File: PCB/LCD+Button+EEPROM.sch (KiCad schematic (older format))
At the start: 17 parts, among them J2 Conn_01x03, J3 Conn_01x04, J4 Conn_01x03, J5 Conn_01x04, J6 Conn_01x04, SW1 B1, SW2 B2, SW3 B3, SW4 B4, SW5 B5, SW6 B6, U4 24LC256

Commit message: Footprint Assigned
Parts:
- C18: footprint (none) -> Capacitor_SMD:C_0805_2012Metric
- J2, J4: footprint (none) -> Connector_PinHeader_2.54mm:PinHeader_1x03_P2.54mm_Vertical
- J3, J5, J6: footprint (none) -> Connector_PinHeader_2.54mm:PinHeader_1x04_P2.54mm_Vertical
- LCD1: footprint (none) -> Kicad Library:OLED_I2C_128x64
- R10, R11: footprint (none) -> Resistor_SMD:R_0805_2012Metric
- RESET1, SW1, SW2, SW3, SW4, SW5, SW6: footprint (none) -> Kicad Library:Push_button_silicon_mute
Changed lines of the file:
@@
 F 0 "RESET1" H 5650 4000 50  0000 R CNN
 F 1 "RESET" H 5875 3950 50  0001 R CNN
-F 2 "" H 5525 4050 50  0001 C CNN
+F 2 "Kicad Library:Push_button_silicon_mute" H 5525 4050 50  0001 C CNN
 F 3 "~" H 5525 4050 50  0001 C CNN
 	1    5525 3850
@@
 F 0 "SW1" H 5600 4250 50  0000 R CNN
 F 1 "B1" H 5725 4200 50  0001 R CNN
-F 2 "" H 5525 4300 50  0001 C CNN
+F 2 "Kicad Library:Push_button_silicon_mute" H 5525 4300 50  0001 C CNN
 F 3 "~" H 5525 4300 50  0001 C CNN
 	1    5525 4100
@@
 F 0 "SW2" H 5600 4500 50  0000 R CNN
 F 1 "B2" H 5725 4450 50  0001 R CNN
-F 2 "" H 5525 4550 50  0001 C CNN
+F 2 "Kicad Library:Push_button_silicon_mute" H 5525 4550 50  0001 C CNN
 F 3 "~" H 5525 4550 50  0001 C CNN
 	1    5525 4350
@@
 F 0 "SW3" H 5600 4750 50  0000 R CNN
 F 1 "B3" H 5725 4700 50  0001 R CNN
-F 2 "" H 5525 4800 50  0001 C CNN
+F 2 "Kicad Library:Push_button_silicon_mute" H 5525 4800 50  0001 C CNN
 F 3 "~" H 5525 4800 50  0001 C CNN
 	1    5525 4600
@@
 F 0 "SW4" H 4625 4175 50  0000 R CNN
 F 1 "B4" H 4725 4125 50  0001 R CNN
-F 2 "" H 4525 4225 50  0001 C CNN
+F 2 "Kicad Library:Push_button_silicon_mute" H 4525 4225 50  0001 C CNN
 F 3 "~" H 4525 4225 50  0001 C CNN
 	1    4525 4025
@@
 F 0 "SW5" H 4625 4425 50  0000 R CNN
 F 1 "B5" H 4725 4375 50  0001 R CNN
-F 2 "" H 4525 4475 50  0001 C CNN
+F 2 "Kicad Library:Push_button_silicon_mute" H 4525 4475 50  0001 C CNN
 F 3 "~" H 4525 4475 50  0001 C CNN
 	1    4525 4275
@@
 F 0 "SW6" H 4625 4675 50  0000 R CNN
 F 1 "B6" H 4725 4625 50  0001 R CNN
-F 2 "" H 4525 4725 50  0001 C CNN
+F 2 "Kicad Library:Push_button_silicon_mute" H 4525 4725 50  0001 C CNN
 F 3 "~" H 4525 4725 50  0001 C CNN
 	1    4525 4525
@@
 F 0 "J3" H 6605 3896 50  0000 L CNN
 F 1 "Conn_01x04" H 6605 3851 50  0001 L CNN
-F 2 "" H 6525 3950 50  0001 C CNN
+F 2 "Connector_PinHeader_2.54mm:PinHeader_1x04_P2.54mm_Vertical" H 6525 3950 50  0001 C CNN
 F 3 "~" H 6525 3950 50  0001 C CNN
 	1    6525 3950
@@
 F 0 "J2" H 3750 4125 50  0000 C CNN
 F 1 "Conn_01x03" H 3518 3891 50  0001 C CNN
-F 2 "" H 3600 4125 50  0001 C CNN
+F 2 "Connector_PinHeader_2.54mm:PinHeader_1x03_P2.54mm_Vertical" H 3600 4125 50  0001 C CNN
 F 3 "~" H 3600 4125 50  0001 C CNN
 	1    3600 4125
@@
 AR Path="/5F734488" Ref="#PWR?"  Part="1"
 AR Path="/5F584CC7/5F734488" Ref="#PWR?"  Part="1"
-AR Path="/5F7200D9/5F734488" Ref="#PWR03"  Part="1"
-F 0 "#PWR03" H 5025 4350 50  0001 C CNN
+AR Path="/5F7200D9/5F734488" Ref="#PWR0101"  Part="1"
+F 0 "#PWR0101" H 5025 4350 50  0001 C CNN
 F 1 "GND" H 5030 4427 50  0000 C CNN
 F 2 "" H 5025 4600 50  0001 C CNN
@@
 F 0 "J5" V 5100 5175 50  0000 C CNN
 F 1 "Conn_01x04" V 5100 5175 50  0001 C CNN
-F 2 "" H 5000 5200 50  0001 C CNN
+F 2 "Connector_PinHeader_2.54mm:PinHeader_1x04_P2.54mm_Vertical" H 5000 5200 50  0001 C CNN
 F 3 "~" H 5000 5200 50  0001 C CNN
 	1    5000 5200
@@
 AR Path="/5F647117" Ref="#PWR?"  Part="1"
 AR Path="/5F584CC7/5F647117" Ref="#PWR?"  Part="1"
-AR Path="/5F7200D9/5F647117" Ref="#PWR02"  Part="1"
-F 0 "#PWR02" H 4900 5425 50  0001 C CNN
+AR Path="/5F7200D9/5F647117" Ref="#PWR0102"  Part="1"
+F 0 "#PWR0102" H 4900 5425 50  0001 C CNN
 F 1 "GND" H 4905 5502 50  0000 C CNN
 F 2 "" H 4900 5675 50  0001 C CNN
@@
 F 0 "J4" V 4650 5200 50  0000 C CNN
 F 1 "Conn_01x03" H 4468 4966 50  0001 C CNN
-F 2 "" H 4550 5200 50  0001 C CNN
+F 2 "Connector_PinHeader_2.54mm:PinHeader_1x03_P2.54mm_Vertical" H 4550 5200 50  0001 C CNN
 F 3 "~" H 4550 5200 50  0001 C CNN
 	1    4550 5200
@@
 F 0 "J6" V 5650 5125 50  0000 L CNN
 F 1 "Conn_01x04" H 5630 5101 50  0001 L CNN
-F 2 "" H 5550 5200 50  0001 C CNN
+F 2 "Connector_PinHeader_2.54mm:PinHeader_1x04_P2.54mm_Vertical" H 5550 5200 50  0001 C CNN
 F 3 "~" H 5550 5200 50  0001 C CNN
 	1    5550 5200
@@
 F 0 "R10" H 5575 2650 50  0000 L CNN
 F 1 "2K2" V 5525 2550 50  0000 L CNN
-F 2 "" V 5455 2625 50  0001 C CNN
+F 2 "Resistor_SMD:R_0805_2012Metric" V 5455 2625 50  0001 C CNN
 F 3 "~" H 5525 2625 50  0001 C CNN
 	1    5525 2625
@@
 F 0 "R11" H 5850 2650 50  0000 L CNN
 F 1 "2K2" V 5800 2550 50  0000 L CNN
-F 2 "" V 5730 2625 50  0001 C CNN
+F 2 "Resistor_SMD:R_0805_2012Metric" V 5730 2625 50  0001 C CNN
 F 3 "~" H 5800 2625 50  0001 C CNN
 	1    5800 2625
@@
 F 0 "C18" H 4315 2971 50  0000 L CNN
 F 1 "100nF" H 4315 2880 50  0000 L CNN
-F 2 "" H 4238 2775 50  0001 C CNN
+F 2 "Capacitor_SMD:C_0805_2012Metric" H 4238 2775 50  0001 C CNN
 F 3 "~" H 4200 2925 50  0001 C CNN
 	1    4200 2925
@@
 F 0 "LCD1" V 3650 2775 50  0000 C CNN
 F 1 "LCD" V 3650 2775 50  0001 C CNN
-F 2 "" H 3550 2800 50  0001 C CNN
+F 2 "Kicad Library:OLED_I2C_128x64" H 3550 2800 50  0001 C CNN
 F 3 "~" H 3550 2800 50  0001 C CNN
 	1    3550 2800

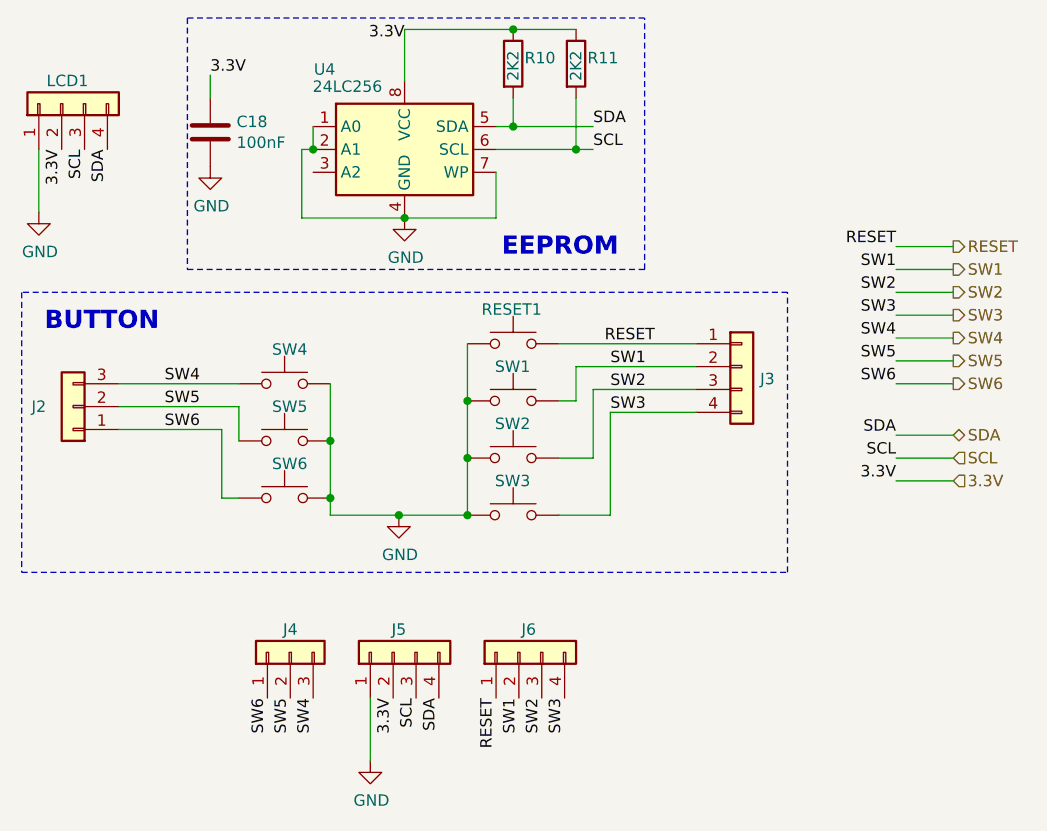
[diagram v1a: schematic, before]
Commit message: Circuit fix (Kicad)
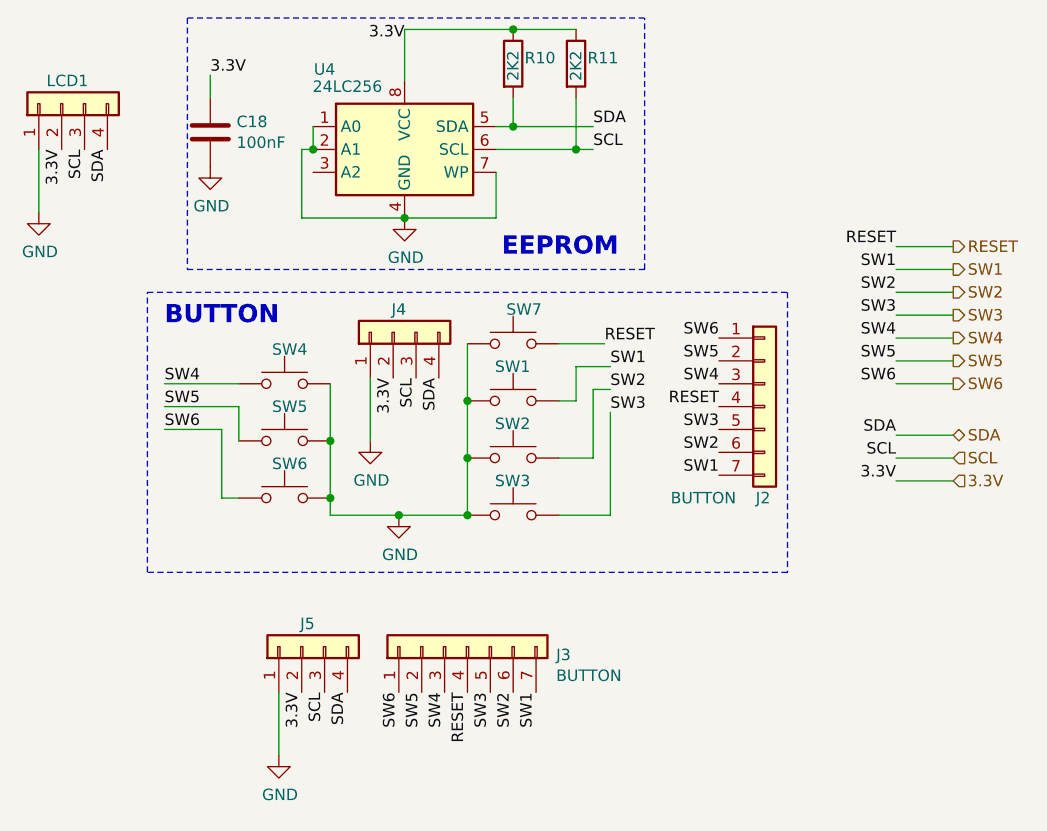
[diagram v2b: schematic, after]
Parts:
- removed J2, J4: Conn_01x03, Connector_PinHeader_2.54mm:PinHeader_1x03_P2.54mm_Vertical, symbol Connector_Generic:Conn_01x03
- removed J3, J6: Conn_01x04, Connector_PinHeader_2.54mm:PinHeader_1x04_P2.54mm_Vertical, symbol Connector_Generic:Conn_01x04
- added J2: BUTTON, Connector_PinSocket_2.54mm:PinSocket_1x07_P2.54mm_Vertical, symbol Connector_Generic:Conn_01x07
- added J3: BUTTON, Connector_PinHeader_2.54mm:PinHeader_1x07_P2.54mm_Vertical, symbol Connector_Generic:Conn_01x07
- added J4: Conn_01x04, Connector_PinHeader_2.54mm:PinHeader_1x04_P2.54mm_Vertical, symbol Connector_Generic:Conn_01x04
- J5: footprint Connector_PinHeader_2.54mm:PinHeader_1x04_P2.54mm_Vertical -> Connector_PinSocket_2.54mm:PinSocket_1x04_P2.54mm_Vertical
- renumbered RESET1 to SW7
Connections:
- net 3.3V: now also J4.2 (Pin_2)
- net GND: now also J4.1 (Pin_1)
- net RESET: now also J2.4 (Pin_4), J3.4 (Pin_4)
- net SCL: now also J4.3 (Pin_3)
- net SDA: now also J4.4 (Pin_4)
- net SW1: now also J2.7 (Pin_7), J3.7 (Pin_7)
- net SW2: now also J2.6 (Pin_6), J3.6 (Pin_6)
- net SW3: now also J2.5 (Pin_5), J3.5 (Pin_5)
- net SW4: now also J2.3 (Pin_3), J3.3 (Pin_3)
- net SW5: now also J2.2 (Pin_2), J3.2 (Pin_2)
- net SW6: now also J2.1 (Pin_1), J3.1 (Pin_1)
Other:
- moved on the sheet: J5
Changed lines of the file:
@@
 P 5525 3850
 AR Path="/5F727D85" Ref="SW?"  Part="1"
-AR Path="/5F7200D9/5F727D85" Ref="RESET1"  Part="1"
-F 0 "RESET1" H 5650 4000 50  0000 R CNN
+AR Path="/5F7200D9/5F727D85" Ref="SW7"  Part="1"
+F 0 "SW7" H 5650 4000 50  0000 R CNN
 F 1 "RESET" H 5875 3950 50  0001 R CNN
 F 2 "Kicad Library:Push_button_silicon_mute" H 5525 4050 50  0001 C CNN
@@
 	1    0    0    -1
 $EndComp
-$Comp
-L Connector_Generic:Conn_01x04 J?
-U 1 1 5F727DAF
-P 6525 3950
-AR Path="/5F727DAF" Ref="J?"  Part="1"
-AR Path="/5F7200D9/5F727DAF" Ref="J3"  Part="1"
-F 0 "J3" H 6605 3896 50  0000 L CNN
-F 1 "Conn_01x04" H 6605 3851 50  0001 L CNN
-F 2 "Connector_PinHeader_2.54mm:PinHeader_1x04_P2.54mm_Vertical" H 6525 3950 50  0001 C CNN
-F 3 "~" H 6525 3950 50  0001 C CNN
-	1    6525 3950
-	1    0    0    -1
-$EndComp
-Wire Wire Line
-	5725 3850 6325 3850
 Wire Wire Line
 	5725 4100 5800 4100
@@
 	5800 4100 5800 3950
 Wire Wire Line
-	5800 3950 6325 3950
-Wire Wire Line
 	5725 4350 5875 4350
 Wire Wire Line
 	5875 4350 5875 4050
 Wire Wire Line
-	5875 4050 6325 4050
-Wire Wire Line
 	5725 4600 5950 4600
 Wire Wire Line
 	5950 4600 5950 4150
 Wire Wire Line
-	5950 4150 6325 4150
-$Comp
-L Connector_Generic:Conn_01x03 J2
-U 1 1 5F72E5D5
-P 3600 4125
-F 0 "J2" H 3750 4125 50  0000 C CNN
-F 1 "Conn_01x03" H 3518 3891 50  0001 C CNN
-F 2 "Connector_PinHeader_2.54mm:PinHeader_1x03_P2.54mm_Vertical" H 3600 4125 50  0001 C CNN
-F 3 "~" H 3600 4125 50  0001 C CNN
-	1    3600 4125
-	-1   0    0    1
-$EndComp
-Wire Wire Line
-	4325 4025 3800 4025
-Wire Wire Line
-	3800 4125 4325 4125
-Wire Wire Line
 	4325 4125 4325 4275
-Wire Wire Line
-	3800 4225 4250 4225
 Wire Wire Line
 	4250 4225 4250 4525
@@
 L Connector_Generic:Conn_01x04 J?
 U 1 1 5F647111
-P 5000 5200
+P 4600 5175
 AR Path="/5F647111" Ref="J?"  Part="1"
 AR Path="/5F7200D9/5F647111" Ref="J5"  Part="1"
-F 0 "J5" V 5100 5175 50  0000 C CNN
-F 1 "Conn_01x04" V 5100 5175 50  0001 C CNN
-F 2 "Connector_PinHeader_2.54mm:PinHeader_1x04_P2.54mm_Vertical" H 5000 5200 50  0001 C CNN
-F 3 "~" H 5000 5200 50  0001 C CNN
-	1    5000 5200
+F 0 "J5" V 4700 5150 50  0000 C CNN
+F 1 "Conn_01x04" V 4700 5150 50  0001 C CNN
+F 2 "Connector_PinSocket_2.54mm:PinSocket_1x04_P2.54mm_Vertical" H 4600 5175 50  0001 C CNN
+F 3 "~" H 4600 5175 50  0001 C CNN
+	1    4600 5175
 	0    -1   -1   0
 $EndComp
@@
 L power:GND #PWR?
 U 1 1 5F647117
-P 4900 5675
+P 4500 5650
 AR Path="/5F647117" Ref="#PWR?"  Part="1"
 AR Path="/5F584CC7/5F647117" Ref="#PWR?"  Part="1"
 AR Path="/5F7200D9/5F647117" Ref="#PWR0102"  Part="1"
-F 0 "#PWR0102" H 4900 5425 50  0001 C CNN
-F 1 "GND" H 4905 5502 50  0000 C CNN
-F 2 "" H 4900 5675 50  0001 C CNN
-F 3 "" H 4900 5675 50  0001 C CNN
-	1    4900 5675
-	1    0    0    -1
-$EndComp
-Wire Wire Line
-	4900 5400 4900 5675
+F 0 "#PWR0102" H 4500 5400 50  0001 C CNN
+F 1 "GND" H 4505 5477 50  0000 C CNN
+F 2 "" H 4500 5650 50  0001 C CNN
+F 3 "" H 4500 5650 50  0001 C CNN
+	1    4500 5650
+	1    0    0    -1
+$EndComp
+Wire Wire Line
+	4500 5375 4500 5650
 Text HLabel 7450 4450 2    50   Input ~ 0
 3.3V
@@
 Text HLabel 7450 4250 2    50   BiDi ~ 0
 SDA
-$Comp
-L Connector_Generic:Conn_01x03 J4
-U 1 1 5F64A1B9
-P 4550 5200
-F 0 "J4" V 4650 5200 50  0000 C CNN
-F 1 "Conn_01x03" H 4468 4966 50  0001 C CNN
-F 2 "Connector_PinHeader_2.54mm:PinHeader_1x03_P2.54mm_Vertical" H 4550 5200 50  0001 C CNN
-F 3 "~" H 4550 5200 50  0001 C CNN
-	1    4550 5200
-	0    -1   -1   0
-$EndComp
-Text Label 4650 5400 3    50   ~ 0
+Text Label 5225 5375 3    50   ~ 0
 SW4
-Text Label 4550 5400 3    50   ~ 0
+Text Label 5125 5375 3    50   ~ 0
 SW5
-Text Label 4450 5400 3    50   ~ 0
+Text Label 5025 5375 3    50   ~ 0
 SW6
-$Comp
-L Connector_Generic:Conn_01x04 J?
-U 1 1 5F64BF4F
-P 5550 5200
-AR Path="/5F64BF4F" Ref="J?"  Part="1"
-AR Path="/5F7200D9/5F64BF4F" Ref="J6"  Part="1"
-F 0 "J6" V 5650 5125 50  0000 L CNN
-F 1 "Conn_01x04" H 5630 5101 50  0001 L CNN
-F 2 "Connector_PinHeader_2.54mm:PinHeader_1x04_P2.54mm_Vertical" H 5550 5200 50  0001 C CNN
-F 3 "~" H 5550 5200 50  0001 C CNN
-	1    5550 5200
-	0    -1   -1   0
-$EndComp
-Text Label 5450 5400 3    50   ~ 0
+Text Label 5325 5375 3    50   ~ 0
 RESET
-Text Label 5550 5400 3    50   ~ 0
+Text Label 5625 5375 3    50   ~ 0
 SW1
-Text Label 5650 5400 3    50   ~ 0
+Text Label 5525 5375 3    50   ~ 0
 SW2
-Text Label 5750 5400 3    50   ~ 0
+Text Label 5425 5375 3    50   ~ 0
 SW3
 $Comp
@@
 Text Label 5875 3000 0    50   ~ 0
 SCL
-Text Label 5000 5400 3    50   ~ 0
-3.3V
-Text Label 5100 5400 3    50   ~ 0
+Text Label 4600 5375 3    50   ~ 0
+3.3V
+Text Label 4700 5375 3    50   ~ 0
 SCL
-Text Label 5200 5400 3    50   ~ 0
+Text Label 4800 5375 3    50   ~ 0
 SDA
 $Comp
@@
 Text Label 3750 3000 3    50   ~ 0
 SDA
-Wire Notes Line
-	6725 3625 3375 3625
-Wire Notes Line
-	3375 3625 3375 4850
-Wire Notes Line
-	3375 4850 6725 4850
-Wire Notes Line
-	6725 4850 6725 3625
-Text Notes 3475 3800 0    79   ~ 16
+Text Notes 4000 3775 0    79   ~ 16
 BUTTON
+$Comp
+L Connector_Generic:Conn_01x07 J3
+U 1 1 5F6D5D8E
+P 5325 5175
+F 0 "J3" V 5289 4787 50  0000 R CNN
+F 1 "BUTTON" V 5198 4787 50  0000 R CNN
+F 2 "Connector_PinHeader_2.54mm:PinHeader_1x07_P2.54mm_Vertical" H 5325 5175 50  0001 C CNN
+F 3 "~" H 5325 5175 50  0001 C CNN
+	1    5325 5175
+	0    -1   -1   0
+$EndComp
+Text Label 6425 4025 2    50   ~ 0
+SW4
+Text Label 6425 3925 2    50   ~ 0
+SW5
+Text Label 6425 3825 2    50   ~ 0
+SW6
+Text Label 6425 4125 2    50   ~ 0
+RESET
+Text Label 6425 4425 2    50   ~ 0
+SW1
+Text Label 6425 4325 2    50   ~ 0
+SW2
+Text Label 6425 4225 2    50   ~ 0
+SW3
+Wire Wire Line
+	5725 3850 5925 3850
+Wire Wire Line
+	5800 3950 5950 3950
+Wire Wire Line
+	5875 4050 5950 4050
+Wire Wire Line
+	4000 4025 4325 4025
+Wire Wire Line
+	4000 4125 4325 4125
+Wire Wire Line
+	4000 4225 4250 4225
+$Comp
+L Connector_Generic:Conn_01x07 J2
+U 1 1 5F6D9CC9
+P 6625 4125
+F 0 "J2" H 6650 3725 50  0000 R CNN
+F 1 "BUTTON" H 6500 3725 50  0000 R CNN
+F 2 "Connector_PinSocket_2.54mm:PinSocket_1x07_P2.54mm_Vertical" H 6625 4125 50  0001 C CNN
+F 3 "~" H 6625 4125 50  0001 C CNN
+	1    6625 4125
+	1    0    0    -1
+$EndComp
+Wire Notes Line
+	6725 3625 6725 4850
+Wire Notes Line
+	6725 4850 3925 4850
+Wire Notes Line
+	3925 4850 3925 3625
+Wire Notes Line
+	3925 3625 6725 3625
+$Comp
+L Connector_Generic:Conn_01x04 J?
+U 1 1 5F7606BF
+P 5000 3800
+AR Path="/5F7606BF" Ref="J?"  Part="1"
+AR Path="/5F7200D9/5F7606BF" Ref="J4"  Part="1"
+F 0 "J4" V 5100 3775 50  0000 C CNN
+F 1 "Conn_01x04" V 5100 3775 50  0001 C CNN
+F 2 "Connector_PinHeader_2.54mm:PinHeader_1x04_P2.54mm_Vertical" H 5000 3800 50  0001 C CNN
+F 3 "~" H 5000 3800 50  0001 C CNN
+	1    5000 3800
+	0    -1   -1   0
+$EndComp
+$Comp
+L power:GND #PWR?
+U 1 1 5F7606C5
+P 4900 4275
+AR Path="/5F7606C5" Ref="#PWR?"  Part="1"
+AR Path="/5F584CC7/5F7606C5" Ref="#PWR?"  Part="1"
+AR Path="/5F7200D9/5F7606C5" Ref="#PWR0113"  Part="1"
+F 0 "#PWR0113" H 4900 4025 50  0001 C CNN
+F 1 "GND" H 4905 4102 50  0000 C CNN
+F 2 "" H 4900 4275 50  0001 C CNN
+F 3 "" H 4900 4275 50  0001 C CNN
+	1    4900 4275
+	1    0    0    -1
+$EndComp
+Wire Wire Line
+	4900 4000 4900 4275
+Text Label 5000 4000 3    50   ~ 0
+3.3V
+Text Label 5100 4000 3    50   ~ 0
+SCL
+Text Label 5200 4000 3    50   ~ 0
+SDA
 $EndSCHEMATC
